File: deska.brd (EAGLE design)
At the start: 55.6 x 83.8 mm, 10 parts

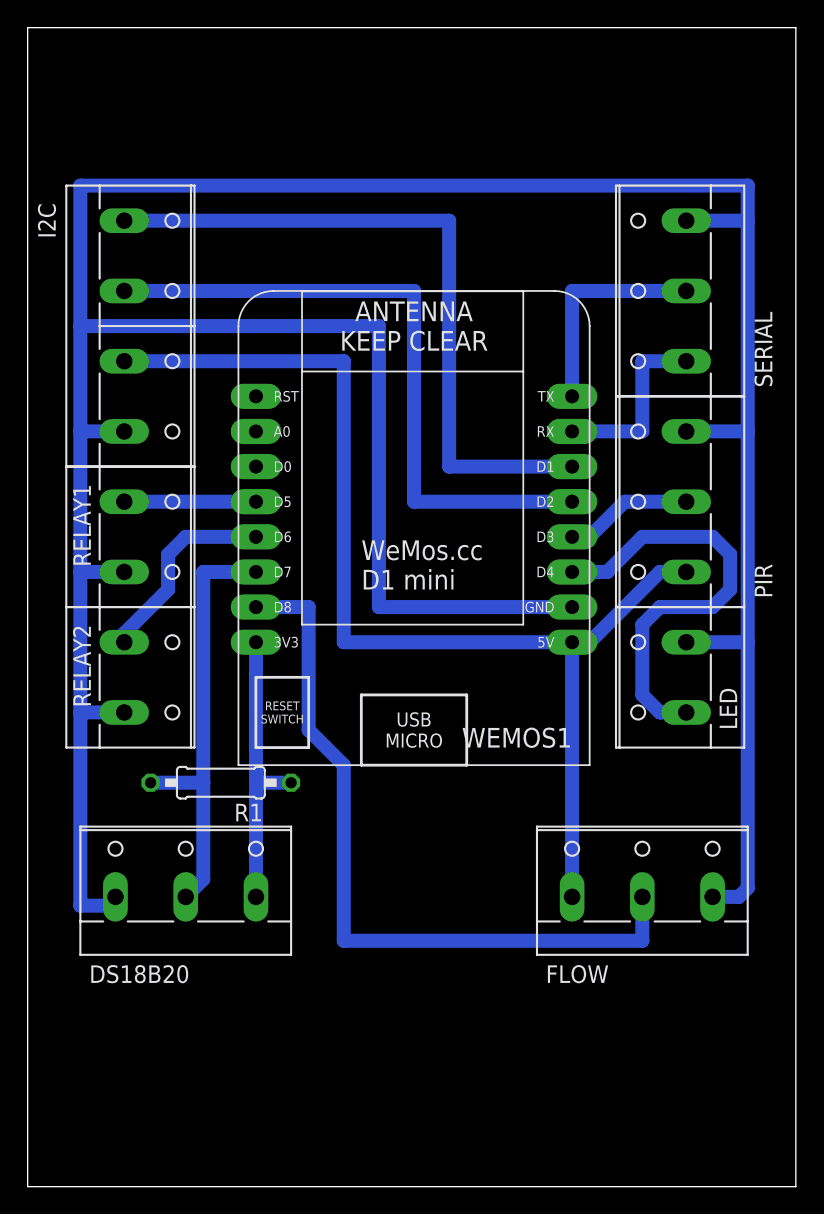
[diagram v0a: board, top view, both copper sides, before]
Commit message: +
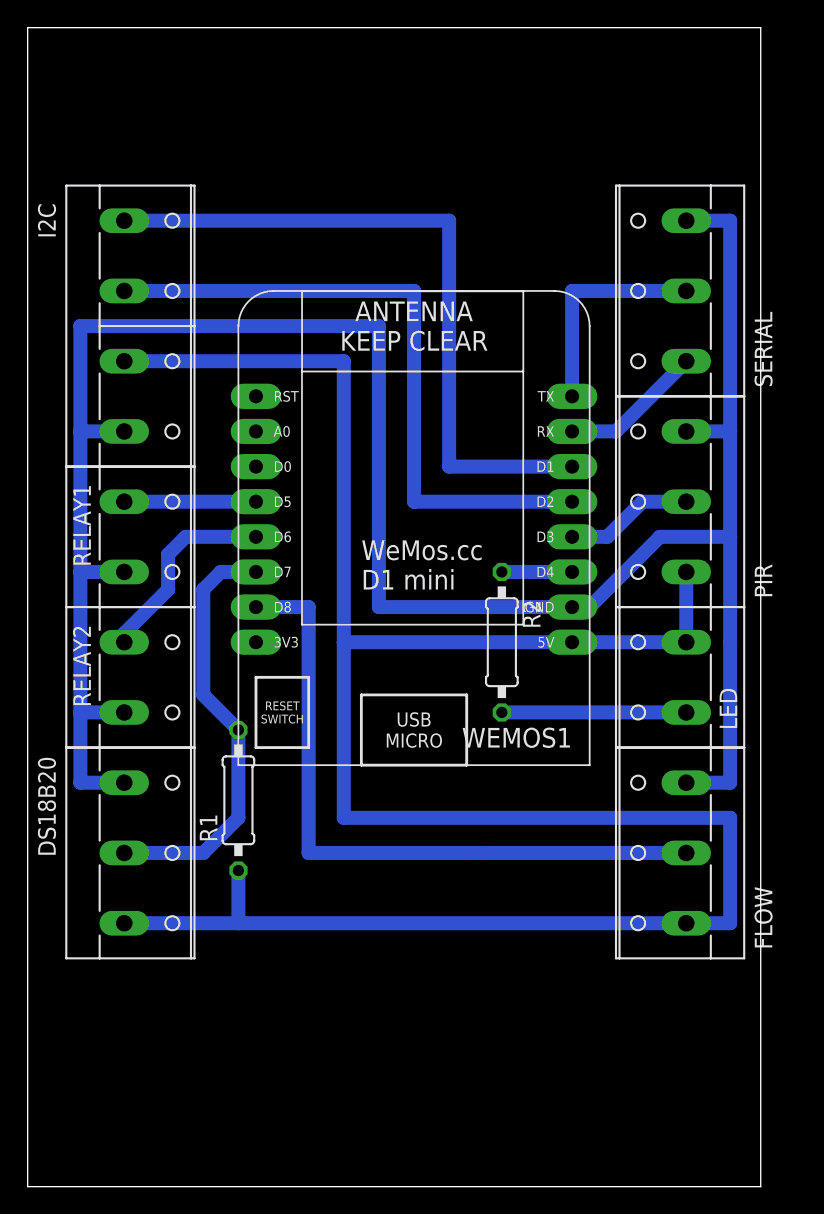
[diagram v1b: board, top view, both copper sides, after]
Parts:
- added R2: 220, rcl:0207/10
- R1: value (none) -> 4k7
- moved DS18B20 4.58 mm to (6.35, 10.2), turned to 270 degrees
- moved FLOW 3.59 mm to (45.7, 10.2), turned to 90 degrees
- moved R1 1.80 mm to (14.0, 14.0), turned to 90 degrees
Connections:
- removed net N$11: DS18B20.3, R1.1, WEMOS1.3V3
- new net N$12: LED.1, R2.2
- net +5V: now also DS18B20.3, LED.2, R1.1
- net GND: no longer LED.2
- net N$6: now also R2.1; no longer LED.1
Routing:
- net +5V: track 81.5 -> 161.9 mm
- net GND: track 235.5 -> 165.3 mm
- net N$6: track 31.7 -> 5.08 mm
- net N$11: track 21.0 -> 0.00 mm
- net N$12: track 0.00 -> 13.3 mm
- net N$10: track 55.0 -> 48.9 mm
- net N$2: track 13.3 -> 10.4 mm
- net N$8: track 15.2 -> 14.5 mm
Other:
- board size 55.6 x 83.8 mm -> 53 x 83.8 mm
